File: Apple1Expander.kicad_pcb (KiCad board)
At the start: 2 copper layers, 102.6 x 112.5 mm, 4 parts

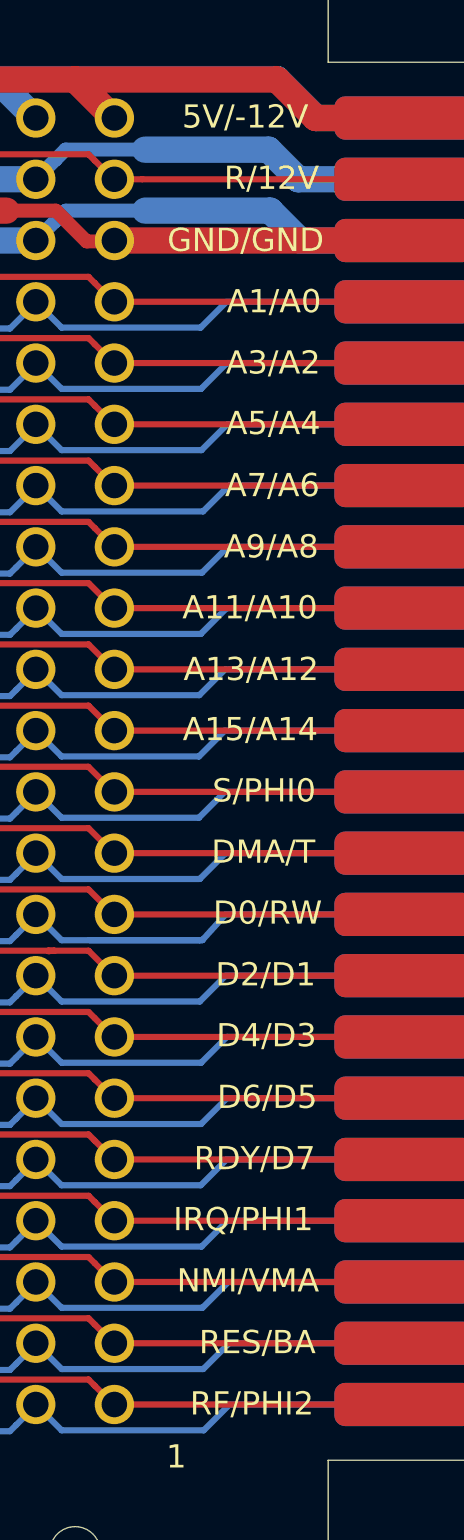
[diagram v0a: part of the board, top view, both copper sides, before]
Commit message: small fixes
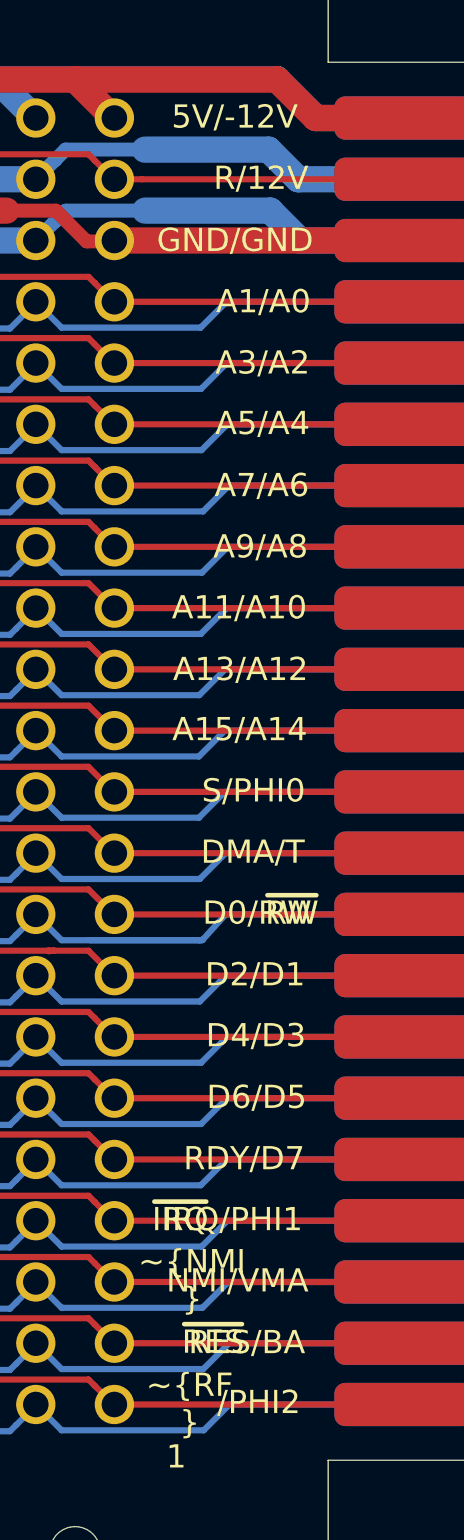
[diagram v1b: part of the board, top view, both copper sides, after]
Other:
- board text added: "/PHI2"
- board text added: "~IRQ"
- board text added: "~NMI"
- board text added: "~RES"
- board text added: "~RF"
- board text added: "~RW"
- board text removed: "RF/PHI2"
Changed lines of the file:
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@@
   (general
     (thickness 1.6)
-    (drawings 44)
+    (drawings 49)
     (tracks 479)
     (zones 0)
@@
     (41 Cmts.User user)
     (42 Eco1.User user)
-    (43 Eco2.User user hide)
+    (43 Eco2.User user)
     (44 Edge.Cuts user)
     (45 Margin user)
@@
     (trace_clearance 0.2)
     (zone_clearance 0.508)
-    (zone_45_only no)
+    (zone_45_only yes)
     (trace_min 0.2)
     (via_size 0.8)
@@
       (outputformat 1)
       (mirror false)
-      (drillshape 1)
+      (drillshape 0)
       (scaleselection 1)
-      (outputdirectory ""))
+      (outputdirectory "/Users/piotrek/Downloads/expander/"))
   )
   (net 0 "")
@@
       (net 22 RF))
   )
+  (gr_text ~RW (at 194.93992 102.59568) (layer F.SilkS)
+    (effects (font (size 1.5 1.5) (thickness 0.3)))
+  )
+  (gr_text ~IRQ (at 187.72632 122.4026) (layer F.SilkS)
+    (effects (font (size 1.5 1.5) (thickness 0.3)))
+  )
+  (gr_text "~NMI\n" (at 188.48324 126.32944) (layer F.SilkS)
+    (effects (font (size 1.5 1.5) (thickness 0.3)))
+  )
+  (gr_text ~RES (at 189.84468 130.32232) (layer F.SilkS)
+    (effects (font (size 1.5 1.5) (thickness 0.3)))
+  )
+  (gr_text "~RF\n" (at 188.32576 134.32028) (layer F.SilkS)
+    (effects (font (size 1.5 1.5) (thickness 0.3)))
+  )
   (gr_text "APPLE-1 PORT EXPANDER" (at 154.559 142.0622) (layer F.SilkS)
     (effects (font (size 1.5 1.5) (thickness 0.3)))
@@
   (gr_line (start 104.394 135.9662) (end 104.394 137.9728) (layer Edge.Cuts) (width 0.05))
   (gr_line (start 104.394 49.6062) (end 104.394 135.9662) (layer Edge.Cuts) (width 0.05))
-  (gr_text 5V/-12V (at 191.9224 51.1302) (layer F.SilkS)
-    (effects (font (size 1.5 1.5) (thickness 0.3)))
-  )
-  (gr_text R/12V (at 193.6242 55.0926) (layer F.SilkS)
-    (effects (font (size 1.5 1.5) (thickness 0.3)))
-  )
-  (gr_text GND/GND (at 191.9478 59.1058) (layer F.SilkS)
-    (effects (font (size 1.5 1.5) (thickness 0.3)))
-  )
-  (gr_text A1/A0 (at 193.7766 63.0682) (layer F.SilkS)
-    (effects (font (size 1.5 1.5) (thickness 0.3)))
-  )
-  (gr_text A3/A2 (at 193.7258 67.0306) (layer F.SilkS)
-    (effects (font (size 1.5 1.5) (thickness 0.3)))
-  )
-  (gr_text A5/A4 (at 193.7258 70.9422) (layer F.SilkS)
-    (effects (font (size 1.5 1.5) (thickness 0.3)))
-  )
-  (gr_text A7/A6 (at 193.675 74.9554) (layer F.SilkS)
-    (effects (font (size 1.5 1.5) (thickness 0.3)))
-  )
-  (gr_text A9/A8 (at 193.5988 78.9178) (layer F.SilkS)
-    (effects (font (size 1.5 1.5) (thickness 0.3)))
-  )
-  (gr_text A11/A10 (at 192.2272 82.8548) (layer F.SilkS)
-    (effects (font (size 1.5 1.5) (thickness 0.3)))
-  )
-  (gr_text A13/A12 (at 192.3034 86.8426) (layer F.SilkS)
-    (effects (font (size 1.5 1.5) (thickness 0.3)))
-  )
-  (gr_text "A15/A14\n" (at 192.2526 90.7288) (layer F.SilkS)
-    (effects (font (size 1.5 1.5) (thickness 0.3)))
-  )
-  (gr_text S/PHI0 (at 193.1424 94.6912) (layer F.SilkS)
-    (effects (font (size 1.5 1.5) (thickness 0.3)))
-  )
-  (gr_text DMA/T (at 193.0908 98.6536) (layer F.SilkS)
-    (effects (font (size 1.5 1.5) (thickness 0.3)))
-  )
-  (gr_text D0/RW (at 193.3702 102.5906) (layer F.SilkS)
-    (effects (font (size 1.5 1.5) (thickness 0.3)))
-  )
-  (gr_text D2/D1 (at 193.2432 106.5784) (layer F.SilkS)
-    (effects (font (size 1.5 1.5) (thickness 0.3)))
-  )
-  (gr_text D4/D3 (at 193.294 110.5154) (layer F.SilkS)
-    (effects (font (size 1.5 1.5) (thickness 0.3)))
-  )
-  (gr_text "D6/D5\n" (at 193.3448 114.5032) (layer F.SilkS)
-    (effects (font (size 1.5 1.5) (thickness 0.3)))
-  )
-  (gr_text RDY/D7 (at 192.532 118.4656) (layer F.SilkS)
-    (effects (font (size 1.5 1.5) (thickness 0.3)))
-  )
-  (gr_text IRQ/PHI1 (at 191.7954 122.4026) (layer F.SilkS)
-    (effects (font (size 1.5 1.5) (thickness 0.3)))
-  )
-  (gr_text "NMI/VMA\n" (at 192.1002 126.365) (layer F.SilkS)
-    (effects (font (size 1.5 1.5) (thickness 0.3)))
-  )
-  (gr_text RES/BA (at 192.7098 130.3528) (layer F.SilkS)
-    (effects (font (size 1.5 1.5) (thickness 0.3)))
-  )
-  (gr_text RF/PHI2 (at 192.3542 134.3152) (layer F.SilkS)
+  (gr_text 5V/-12V (at 191.24168 51.1302) (layer F.SilkS)
+    (effects (font (size 1.5 1.5) (thickness 0.3)))
+  )
+  (gr_text R/12V (at 192.94348 55.0926) (layer F.SilkS)
+    (effects (font (size 1.5 1.5) (thickness 0.3)))
+  )
+  (gr_text GND/GND (at 191.26708 59.1058) (layer F.SilkS)
+    (effects (font (size 1.5 1.5) (thickness 0.3)))
+  )
+  (gr_text A1/A0 (at 193.09588 63.0682) (layer F.SilkS)
+    (effects (font (size 1.5 1.5) (thickness 0.3)))
+  )
+  (gr_text A3/A2 (at 193.04508 67.0306) (layer F.SilkS)
+    (effects (font (size 1.5 1.5) (thickness 0.3)))
+  )
+  (gr_text A5/A4 (at 193.04508 70.9422) (layer F.SilkS)
+    (effects (font (size 1.5 1.5) (thickness 0.3)))
+  )
+  (gr_text A7/A6 (at 192.99428 74.9554) (layer F.SilkS)
+    (effects (font (size 1.5 1.5) (thickness 0.3)))
+  )
+  (gr_text A9/A8 (at 192.91808 78.9178) (layer F.SilkS)
+    (effects (font (size 1.5 1.5) (thickness 0.3)))
+  )
+  (gr_text A11/A10 (at 191.54648 82.8548) (layer F.SilkS)
+    (effects (font (size 1.5 1.5) (thickness 0.3)))
+  )
+  (gr_text A13/A12 (at 191.62268 86.8426) (layer F.SilkS)
+    (effects (font (size 1.5 1.5) (thickness 0.3)))
+  )
+  (gr_text "A15/A14\n" (at 191.57188 90.7288) (layer F.SilkS)
+    (effects (font (size 1.5 1.5) (thickness 0.3)))
+  )
+  (gr_text S/PHI0 (at 192.46168 94.6912) (layer F.SilkS)
+    (effects (font (size 1.5 1.5) (thickness 0.3)))
+  )
+  (gr_text DMA/T (at 192.41008 98.6536) (layer F.SilkS)
+    (effects (font (size 1.5 1.5) (thickness 0.3)))
+  )
+  (gr_text D0/RW (at 192.68948 102.5906) (layer F.SilkS)
+    (effects (font (size 1.5 1.5) (thickness 0.3)))
+  )
+  (gr_text D2/D1 (at 192.56248 106.5784) (layer F.SilkS)
+    (effects (font (size 1.5 1.5) (thickness 0.3)))
+  )
+  (gr_text D4/D3 (at 192.61328 110.5154) (layer F.SilkS)
+    (effects (font (size 1.5 1.5) (thickness 0.3)))
+  )
+  (gr_text "D6/D5\n" (at 192.66408 114.5032) (layer F.SilkS)
+    (effects (font (size 1.5 1.5) (thickness 0.3)))
+  )
+  (gr_text RDY/D7 (at 191.85128 118.4656) (layer F.SilkS)
+    (effects (font (size 1.5 1.5) (thickness 0.3)))
+  )
+  (gr_text IRQ/PHI1 (at 191.11468 122.4026) (layer F.SilkS)
+    (effects (font (size 1.5 1.5) (thickness 0.3)))
+  )
+  (gr_text "NMI/VMA\n" (at 191.41948 126.365) (layer F.SilkS)
+    (effects (font (size 1.5 1.5) (thickness 0.3)))
+  )
+  (gr_text RES/BA (at 192.02908 130.3528) (layer F.SilkS)
+    (effects (font (size 1.5 1.5) (thickness 0.3)))
+  )
+  (gr_text /PHI2 (at 192.80632 134.22376) (layer F.SilkS)
     (effects (font (size 1.5 1.5) (thickness 0.3)))
   )
@@
   (segment (start 180.322399 57.193001) (end 185.453999 57.193001) (width 0.9) (layer B.Cu) (net 44))
   (segment (start 179.659399 57.856001) (end 180.322399 57.193001) (width 0.9) (layer B.Cu) (net 44))
+  (zone (net 0) (net_name "") (layer B.Mask) (hatch edge 0.508)
+    (connect_pads (clearance 0.508))
+    (min_thickness 0)
+    (fill yes (arc_segments 32) (thermal_gap 0.508) (thermal_bridge_width 0.508))
+    (polygon
+      (pts
+        (xy 207.0354 137.96772) (xy 197.2818 137.96772) (xy 197.2818 47.59452) (xy 207.0354 47.59452)
+      )
+    )
+  )
+  (zone (net 0) (net_name "") (layer F.Mask) (hatch edge 0.508)
+    (connect_pads (clearance 0.508))
+    (min_thickness 0)
+    (fill yes (arc_segments 32) (thermal_gap 0.508) (thermal_bridge_width 0.508))
+    (polygon
+      (pts
+        (xy 207.05064 137.967721) (xy 197.29704 137.967721) (xy 197.29704 47.594521) (xy 207.05064 47.594521)
+      )
+    )
+  )
 )
